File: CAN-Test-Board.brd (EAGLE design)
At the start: 54.6 x 65.7 mm, 51 parts, among them Y1 ECS-80-S-4X, Y2 ECS-80-S-4X

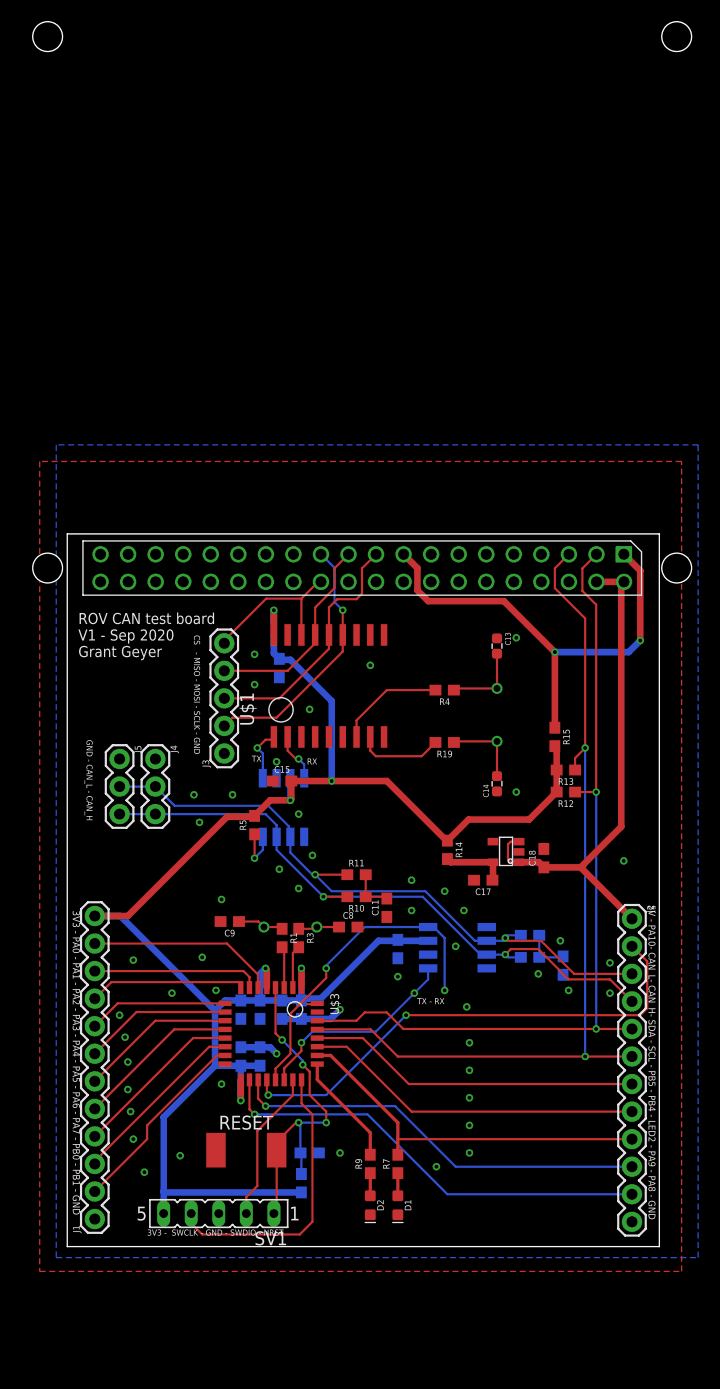
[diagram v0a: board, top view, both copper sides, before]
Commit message: smaller
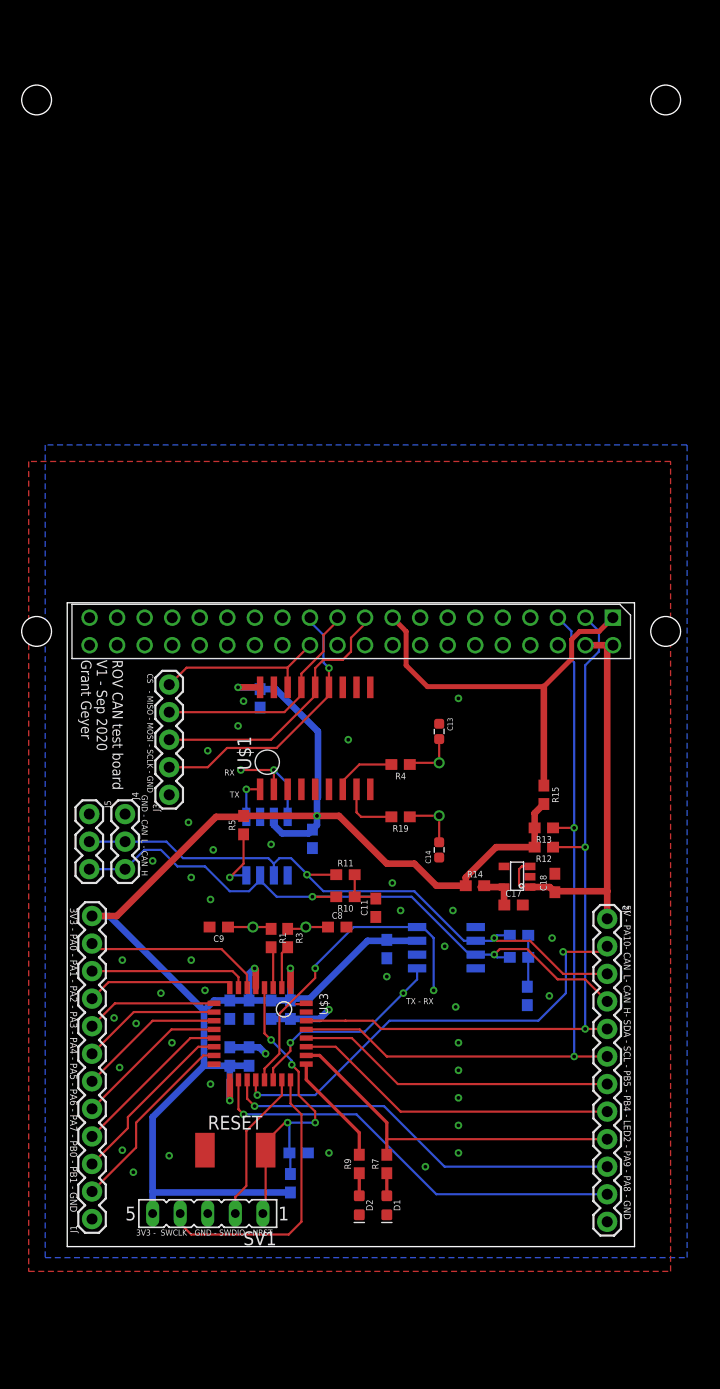
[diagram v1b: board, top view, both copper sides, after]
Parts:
- moved C13 9.51 mm to (34.3, 47.5)
- moved Y2 8.69 mm to (34.3, 42.2)
- moved C14 8.10 mm to (34.3, 36.6)
- moved R19 7.97 mm to (30.7, 39.6)
- moved R4 7.97 mm to (30.7, 44.5)
- moved J3 6.35 mm to (9.40, 41.7)
- moved C15 6.02 mm to (22.6, 37.6), flipped to the bottom, turned to 90 degrees
- moved PCB1 5.93 mm to (58.7, 109.2)
- moved J4 5.80 mm to (5.33, 39.9)
- moved J5 5.80 mm to (2.03, 39.9)
- moved R13 5.71 mm to (43.9, 38.6)
- moved R12 5.47 mm to (43.9, 36.8)
- moved R15 5.43 mm to (43.9, 41.7)
- moved U$1 4.99 mm to (27.9, 42.2)
- moved C16 4.33 mm to (42.4, 23.1)
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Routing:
- net SCL: track 80.5 -> 71.8 mm
- net 5V: track 46.8 -> 39.1 mm
- net SDA: track 76.7 -> 70.0 mm
- net 3V3_PI: track 42.7 -> 37.6 mm, vias 2 -> 0
- net CAN_RX_PI: track 4.59 -> 9.67 mm, vias 1 -> 2
- net OSC2: track 9.96 -> 5.88 mm
- net PA10: track 46.0 -> 42.0 mm
- net OSC1: track 8.01 -> 5.51 mm
- net MISO: track 18.9 -> 21.4 mm
- net N$3: track 7.24 -> 4.96 mm
- net MOSI: track 23.1 -> 25.3 mm
- net 3V3: track 169.5 -> 167.5 mm, vias 6 -> 5
- net N$4: track 7.22 -> 5.19 mm
- net 3V3_REG: track 6.00 -> 4.13 mm
- net SCLK: track 23.6 -> 25.4 mm
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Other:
- board size 54.6 x 65.7 mm -> 52.3 x 59.4 mm
